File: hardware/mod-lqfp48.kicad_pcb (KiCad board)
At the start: 2 copper layers, 2 parts, among them J1 Target, U1 STM32F103C8Tx

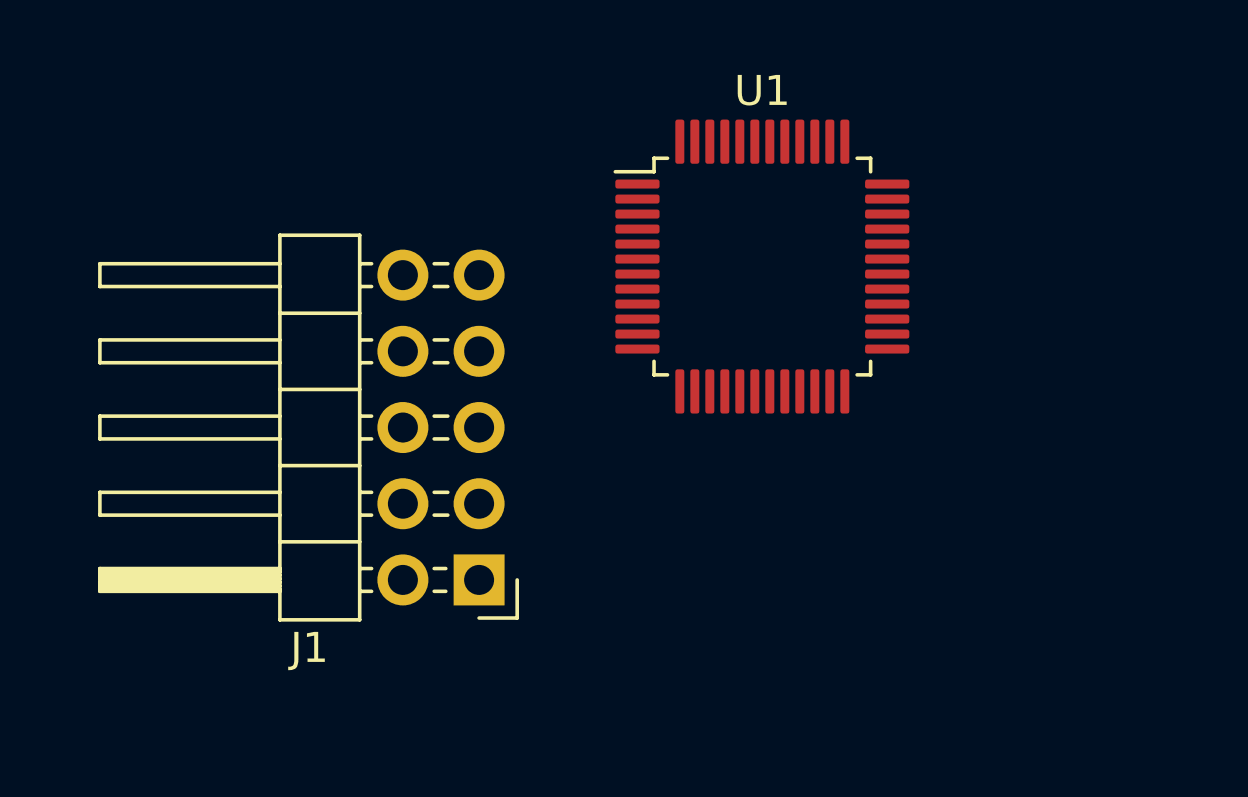
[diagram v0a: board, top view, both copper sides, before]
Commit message: mod-lqfp48 board WIP
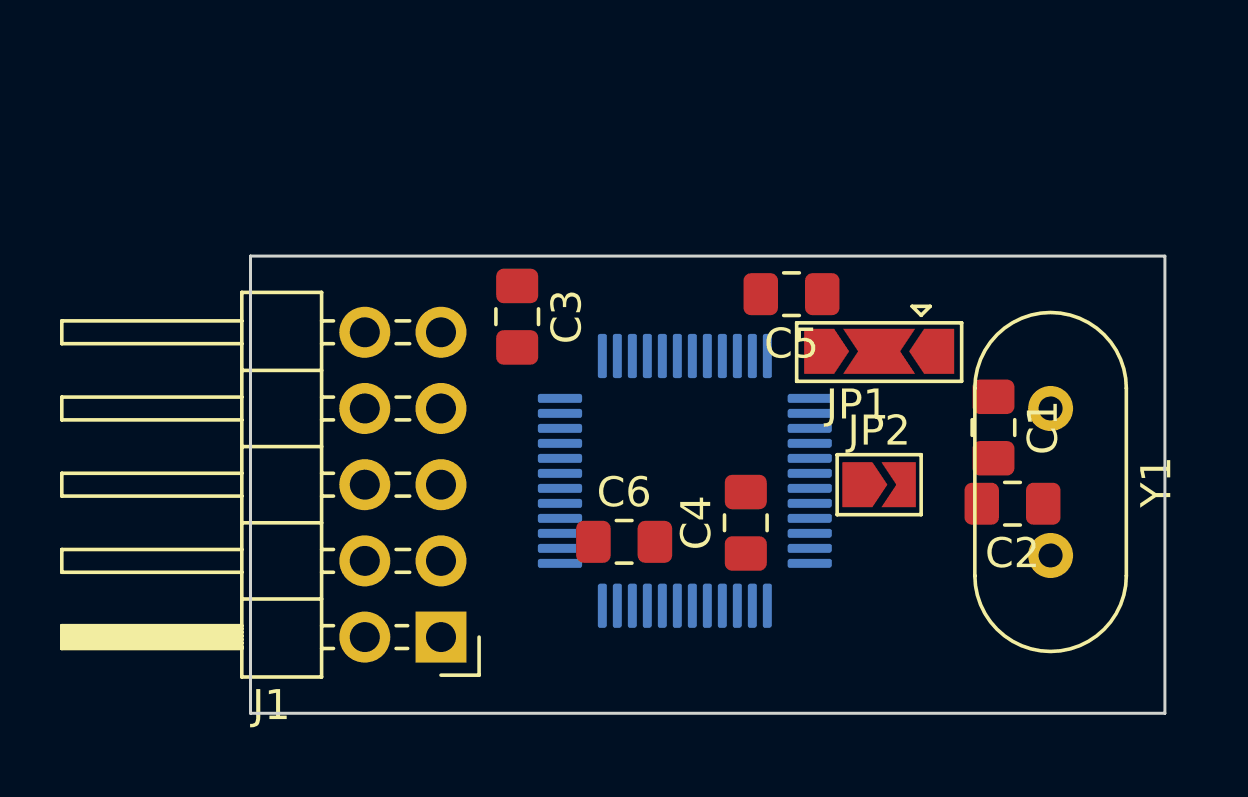
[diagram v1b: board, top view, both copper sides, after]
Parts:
- added C1: 22pF, Capacitor_SMD:C_0805_2012Metric_Pad1.15x1.40mm_HandSolder, F.Cu at (102.2, 94.6)
- added C2: 22pF, Capacitor_SMD:C_0805_2012Metric_Pad1.15x1.40mm_HandSolder, F.Cu at (102.9, 97.2)
- added C3: 100nF, Capacitor_SMD:C_0805_2012Metric_Pad1.15x1.40mm_HandSolder, F.Cu at (86.4, 90.9)
- added C4: 100nF, Capacitor_SMD:C_0805_2012Metric_Pad1.15x1.40mm_HandSolder, F.Cu at (94.0, 97.8)
- added C5: 100nF, Capacitor_SMD:C_0805_2012Metric_Pad1.15x1.40mm_HandSolder, F.Cu at (95.5, 90.2)
- added C6: 100nF, Capacitor_SMD:C_0805_2012Metric_Pad1.15x1.40mm_HandSolder, F.Cu at (89.9, 98.4)
- added JP1: SolderJumper_3_Open, Jumper:SolderJumper-3_P2.0mm_Open_TrianglePad1.0x1.5mm, F.Cu at (98.4, 92.1)
- added JP2: SolderJumper_2_Open, Jumper:SolderJumper-2_P1.3mm_Open_TrianglePad1.0x1.5mm, F.Cu at (98.4, 96.5)
- added Y1: 8MHz, Crystal:Crystal_HC18-U_Vertical, F.Cu at (104.1, 94.0)
- U1: moved to B.Cu
- moved U1 7.60 mm to (91.9, 96.4), turned to 90 degrees
- moved J1 2.29 mm to (83.8, 101.6)
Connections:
- net /VCC renamed +3V3
- J1 pad 1: /USB_DM -> /TX
- J1 pad 10: /RX -> /USB_D-
- J1 pad 2: /USB_DP -> /RX
- J1 pad 7: /SWDIO -> /SWCLK
- J1 pad 8: /SWCLK -> /SWDIO
- J1 pad 9: /TX -> /USB_D+
- U1 pad 32: /USB_DM -> /USB_D-
- U1 pad 33: /USB_DP -> /USB_D+
- U1 pad 5: /CLK -> Net-(JP1-Pad2)
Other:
- board outline added: 30.5 x 15.2 mm
